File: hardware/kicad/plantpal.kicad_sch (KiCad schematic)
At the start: 0 parts

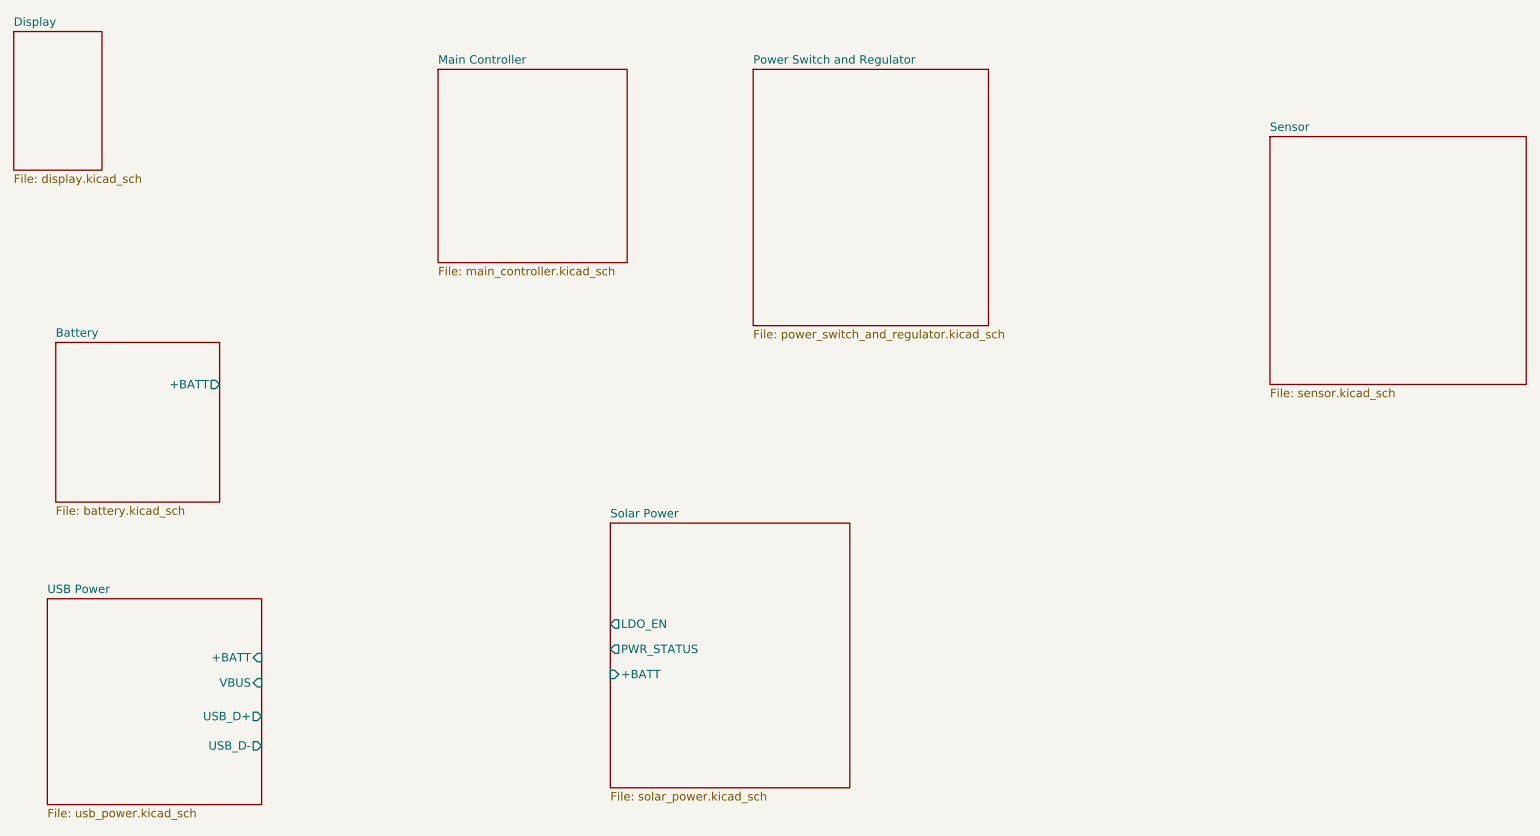
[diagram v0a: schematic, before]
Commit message: schematic restructure update
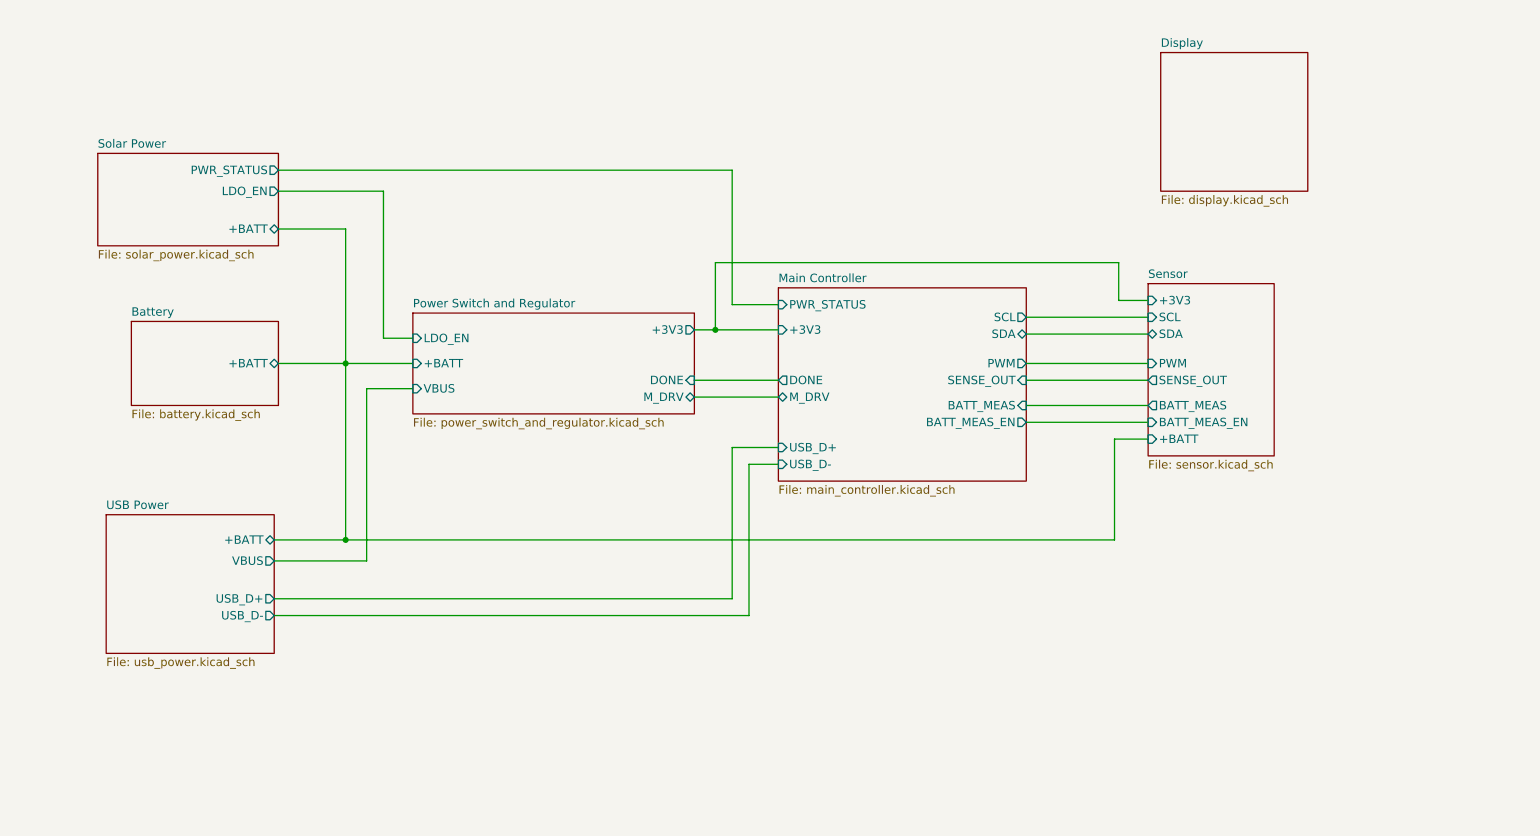
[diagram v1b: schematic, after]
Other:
- sheet Main Controller ports: added +3V3, BATT_MEAS, BATT_MEAS_EN, DONE, M_DRV, PWM, PWR_STATUS, SCL, SDA, SENSE_OUT, USB_D+, USB_D-; removed none
- sheet Power Switch and Regulator ports: added +3V3, +BATT, DONE, LDO_EN, M_DRV, VBUS; removed none
- sheet Sensor ports: added +3V3, +BATT, BATT_MEAS, BATT_MEAS_EN, PWM, SCL, SDA, SENSE_OUT; removed none
